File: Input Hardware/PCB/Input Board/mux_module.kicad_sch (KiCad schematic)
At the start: 2 parts

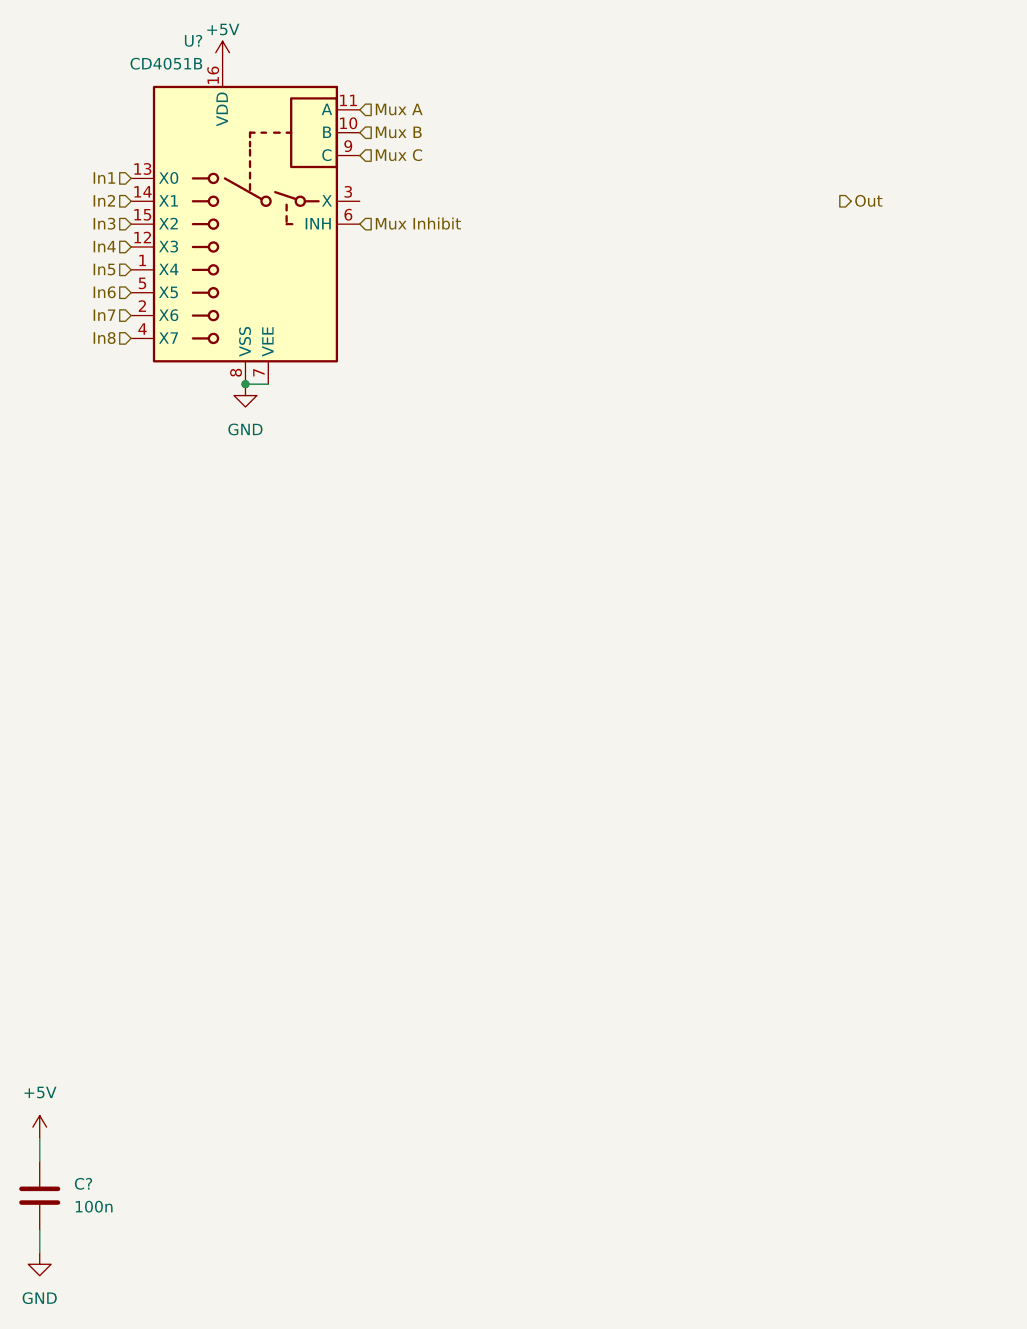
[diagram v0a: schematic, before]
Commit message: Progress
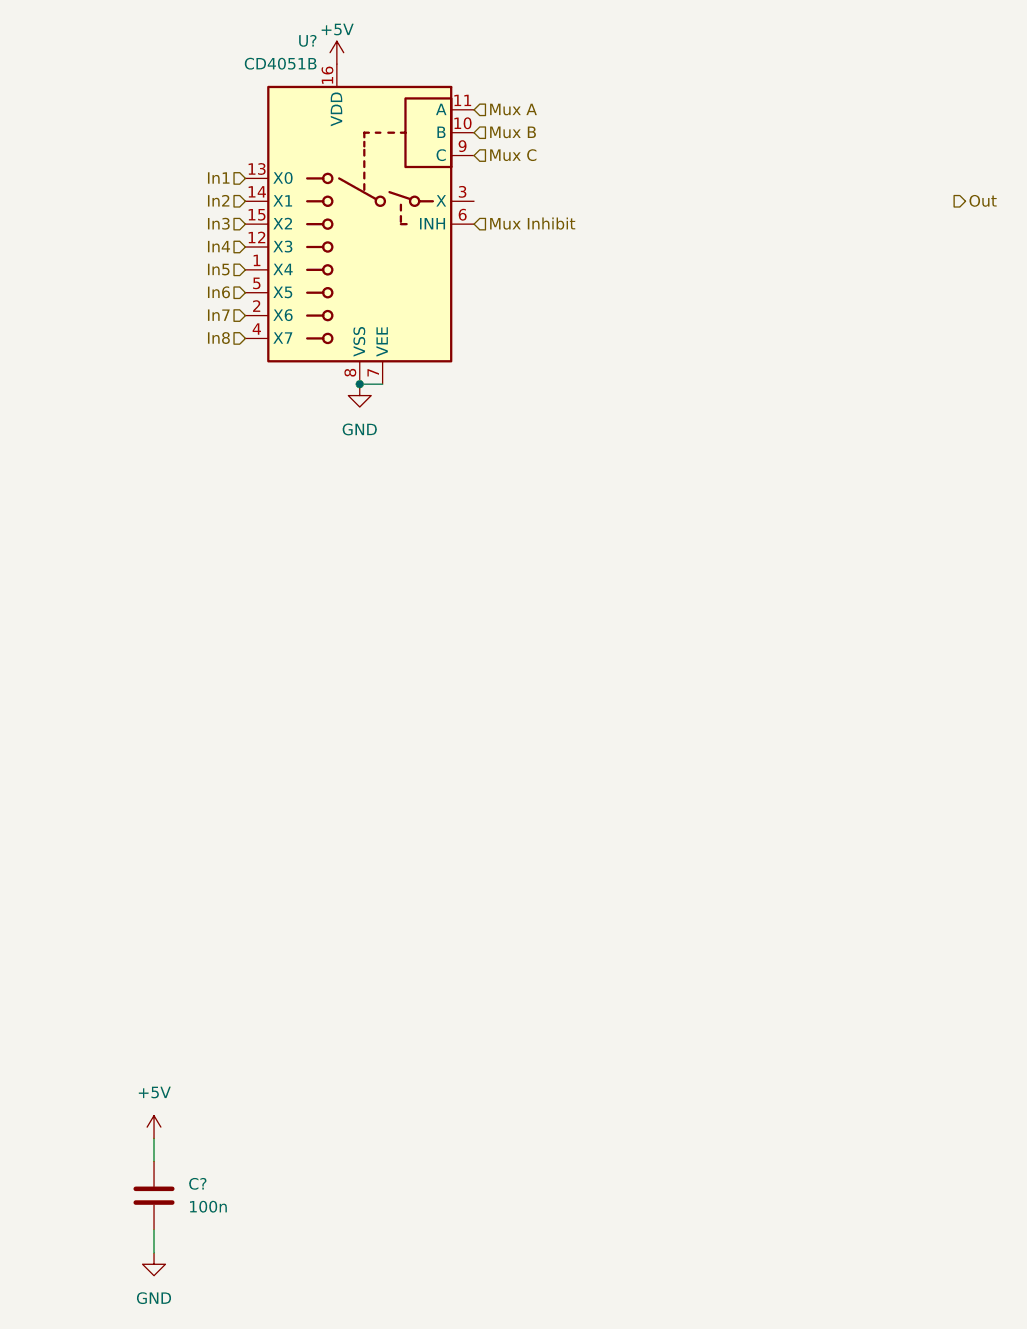
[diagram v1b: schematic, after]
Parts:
- removed C?: 100n, Capacitor_SMD:C_0603_1608Metric, symbol Device:C
- removed U?: CD4051B, symbol Analog_Switch:CD4051B
- added C?: 100n, Capacitor_SMD:C_0603_1608Metric, symbol Device:C
- added U?: CD4051B, symbol Analog_Switch:CD4051B
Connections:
- net +5V: now also C?.1, U?.16 (VDD)
- net GND: now also C?.2, U?.7 (VEE), U?.8 (VSS)
- net In1: now also U?.13 (X0)
- net In2: now also U?.14 (X1)
- net In3: now also U?.15 (X2)
- net In4: now also U?.12 (X3)
- net In5: now also U?.1 (X4)
- net In6: now also U?.5 (X5)
- net In7: now also U?.2 (X6)
- net In8: now also U?.4 (X7)
- net Mux A: now also U?.11 (A)
- net Mux B: now also U?.10 (B)
- net Mux C: now also U?.9 (C)
- net Mux Inhibit: now also U?.6 (INH)
